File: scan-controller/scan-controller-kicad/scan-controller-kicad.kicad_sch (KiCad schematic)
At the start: 36 parts, among them CN1 24V in, J1 FTDI, J5 ICSP, J6 Raspi UART, J7 Raspi GPIO, Q2 IRLML2502, Q3 IRLML6402, SW3 Reset, U5 ATmega328P, Y1 8MHz

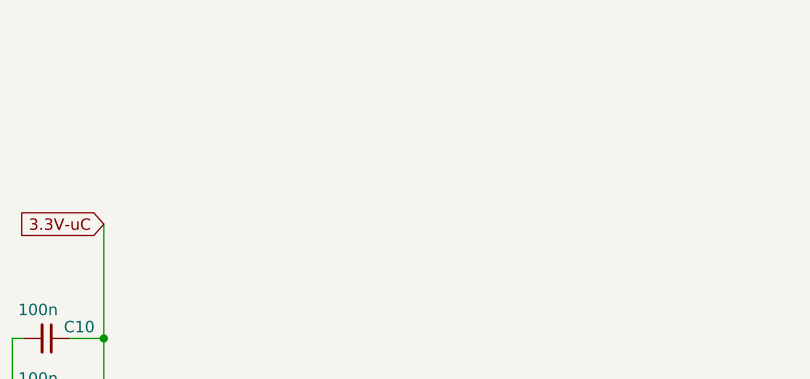
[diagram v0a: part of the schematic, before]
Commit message: minor layout tweaks, todos
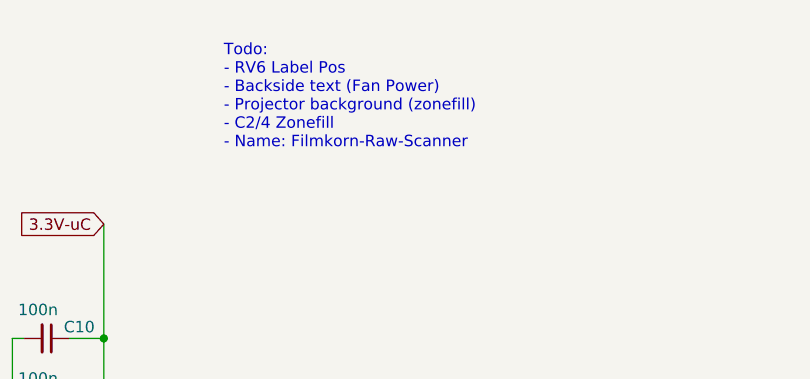
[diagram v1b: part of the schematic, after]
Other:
- note added: "Todo: - RV6 Label Pos - Backside text (Fan Power) - Projector background (zonefill) - C2/4 Zonefill - Name: Filmkorn-Raw-Scanner"
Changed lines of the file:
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@@
     (effects (font (size 1 1)) (justify left bottom))
+  )
+  (text "Todo:\n- RV6 Label Pos\n- Backside text (Fan Power)\n- Projector background (zonefill)\n- C2/4 Zonefill\n- Name: Filmkorn-Raw-Scanner\n"
+    (at 201.93 29.845 0)
+    (effects (font (size 1.27 1.27)) (justify left bottom))
   )
   (label "GNDD" (at 64.135 42.545 0) (fields_autoplaced)

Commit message: Cosmetic PCB Changes (not in sync with netlist yet)
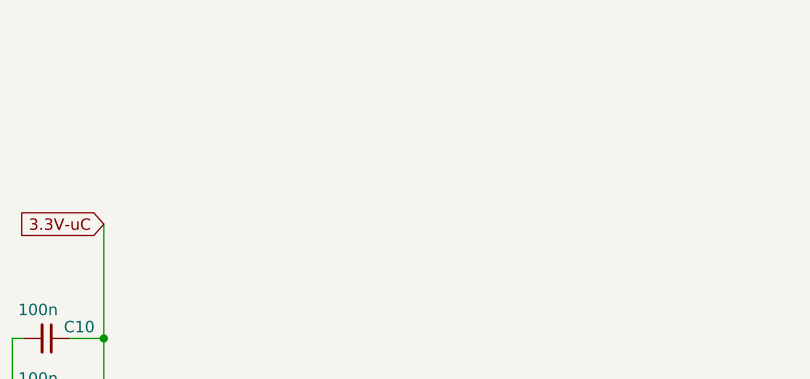
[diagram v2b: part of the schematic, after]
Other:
- note removed: "Todo: - RV6 Label Pos - Backside text (Fan Power) - Projector background (zonefill) - C2/4 Zonefill - Name: Filmkorn-Raw-Scanner"
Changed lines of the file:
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@@
     (effects (font (size 1 1)) (justify left bottom))
-  )
-  (text "Todo:\n- RV6 Label Pos\n- Backside text (Fan Power)\n- Projector background (zonefill)\n- C2/4 Zonefill\n- Name: Filmkorn-Raw-Scanner\n"
-    (at 201.93 29.845 0)
-    (effects (font (size 1.27 1.27)) (justify left bottom))
   )
   (label "GNDD" (at 64.135 42.545 0) (fields_autoplaced)
